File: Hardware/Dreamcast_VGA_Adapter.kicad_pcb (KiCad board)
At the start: 2 copper layers, 56.6 x 57.7 mm, 41 parts, among them J1 AudioJack3, J2 DB15_Female_HighDensity_Mount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, J3 Conn_02x08_Odd_Even, SW1 SW_DIP_x02, U1 THS7316, U2 74HCT2G34

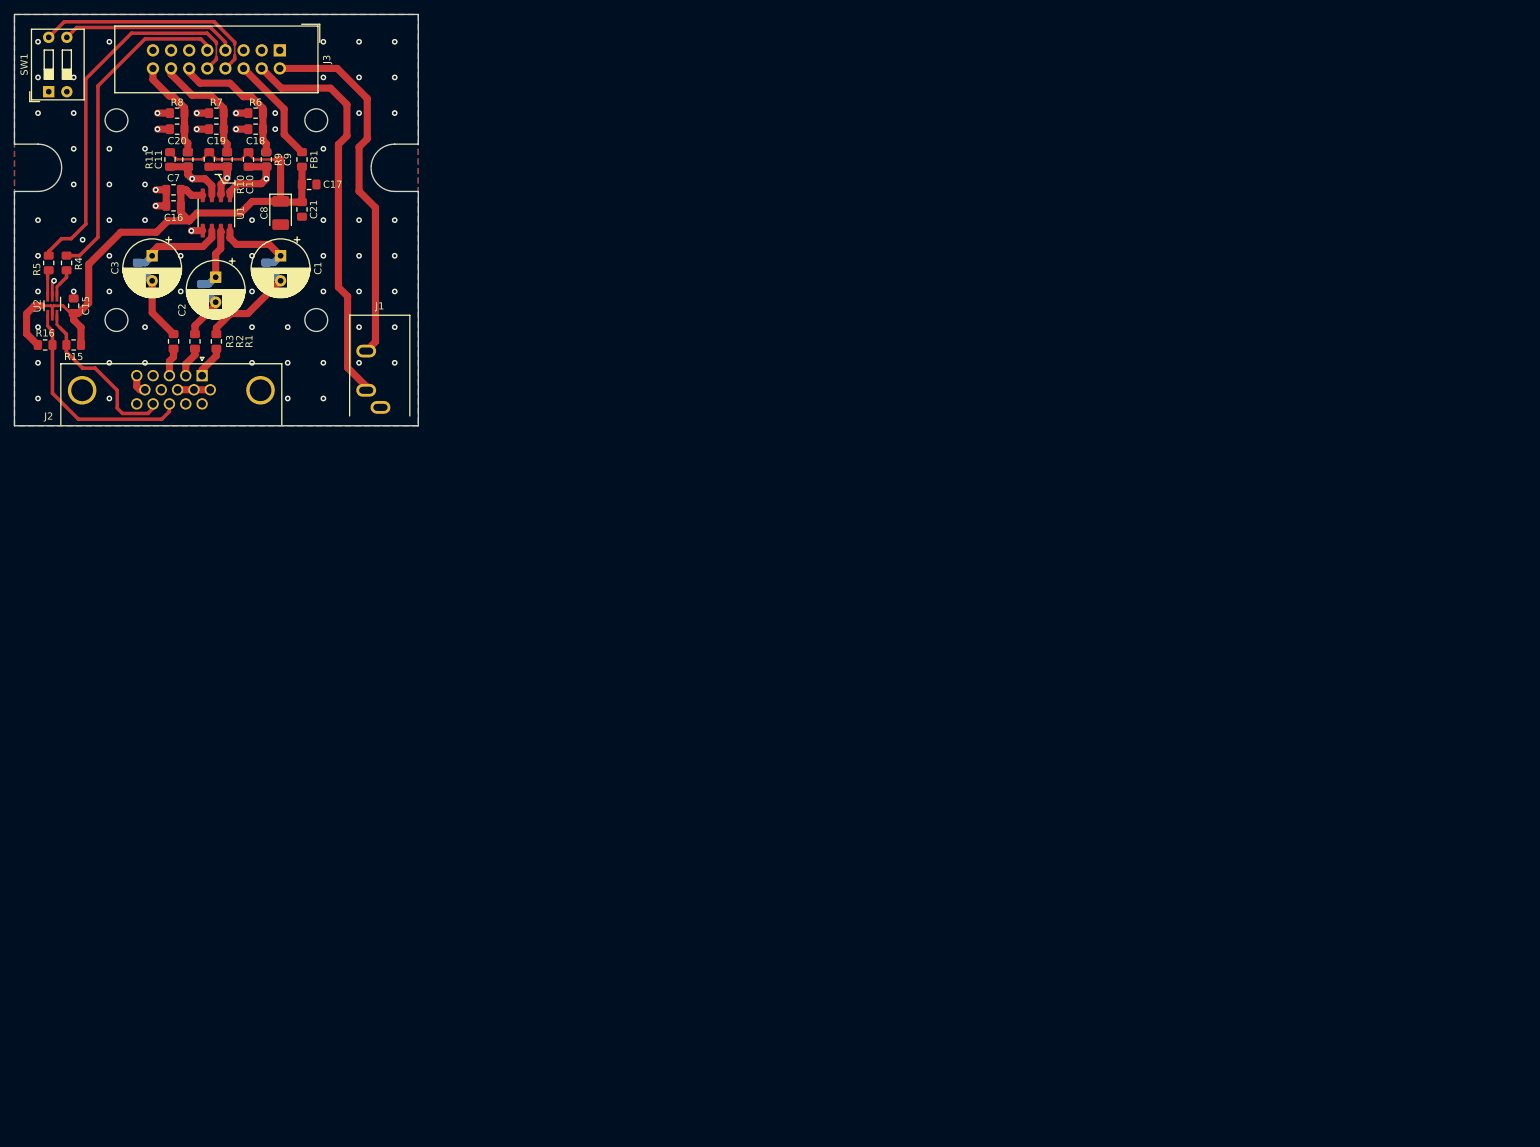
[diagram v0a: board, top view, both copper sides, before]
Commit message: Created 3D model
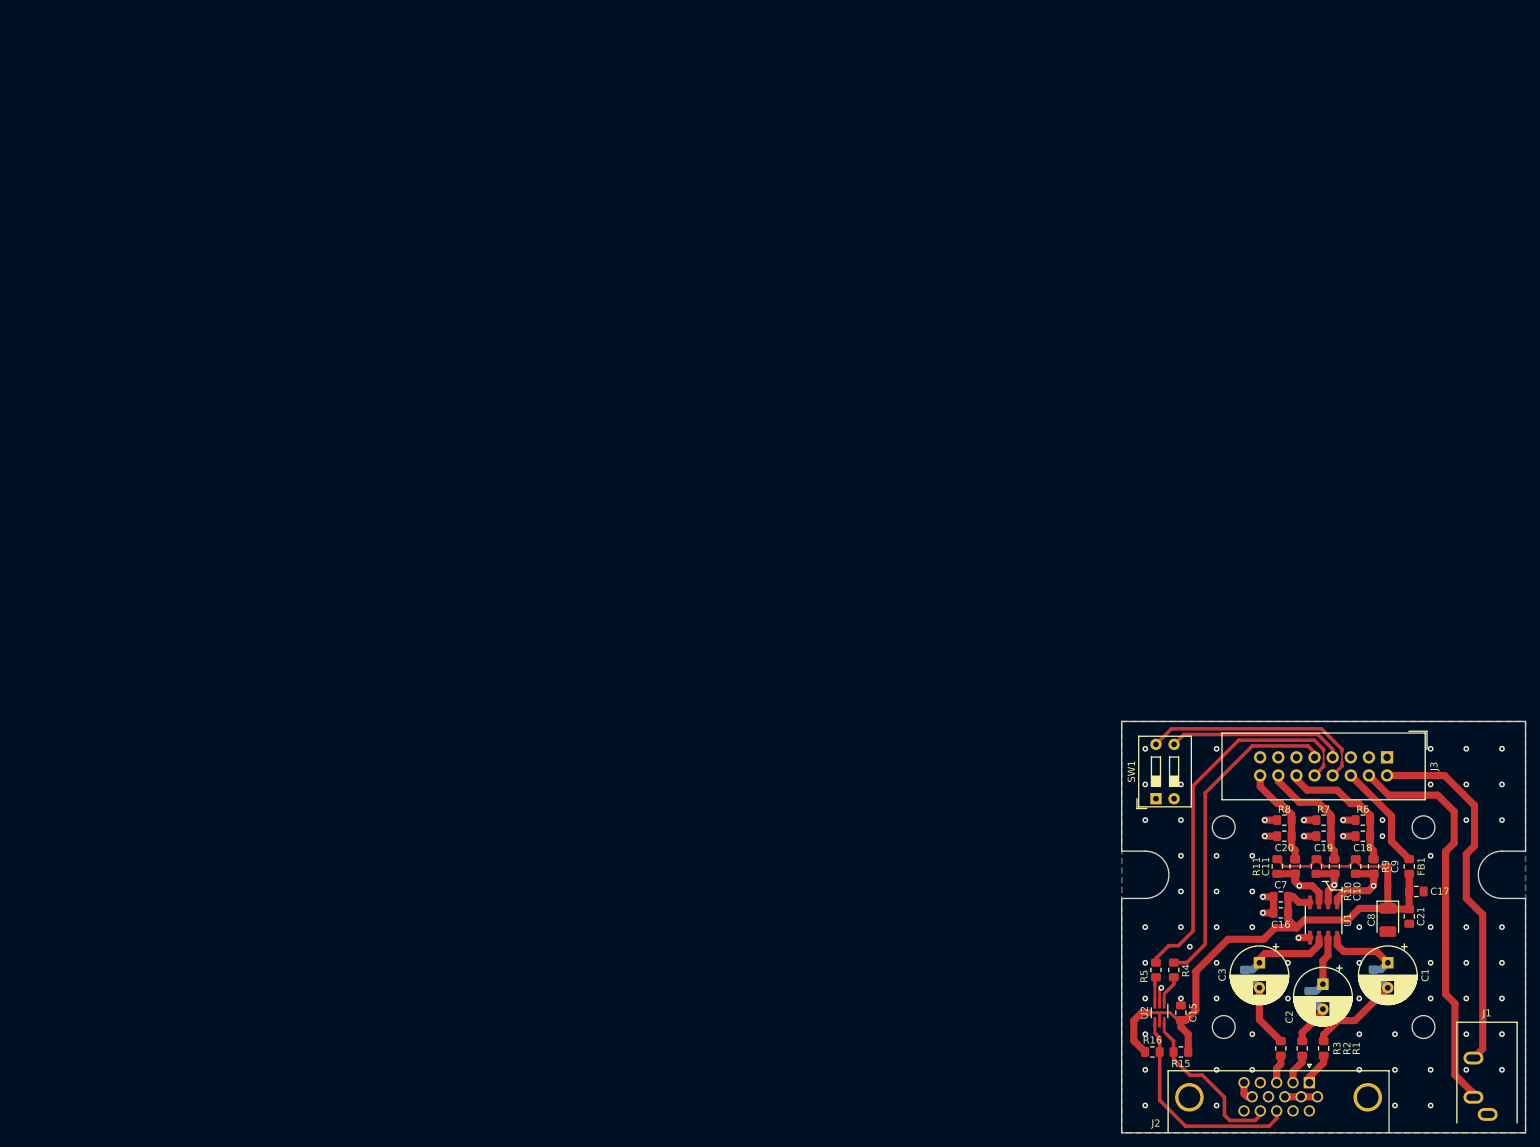
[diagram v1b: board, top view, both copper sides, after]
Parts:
- moved C1 184.1 mm to (164.2, 104.1)
- moved C10 184.1 mm to (156.7, 90.6)
- moved C11 184.1 mm to (151.2, 90.6)
- moved C15 184.1 mm to (135.2, 111.1)
- moved C16 184.1 mm to (149.2, 97.1)
- moved C17 184.1 mm to (168.2, 94.1)
- moved C18 184.1 mm to (160.7, 86.3)
- moved C19 184.1 mm to (155.2, 86.3)
- moved C2 184.1 mm to (155.1, 107.1)
- moved C20 184.1 mm to (149.7, 86.3)
- moved C21 184.1 mm to (167.2, 97.6)
- moved C3 184.1 mm to (146.2, 104.1)
- moved C4 184.1 mm to (162.2, 106.1)
- moved C5 184.1 mm to (153.2, 109.1)
- moved C6 184.1 mm to (144.2, 106.1)
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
